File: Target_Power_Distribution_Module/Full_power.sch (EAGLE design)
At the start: 28 parts, among them IC1 MCP1702, Q1 NFET, Q2 PFET, Q3 NFET, Q4 PFET

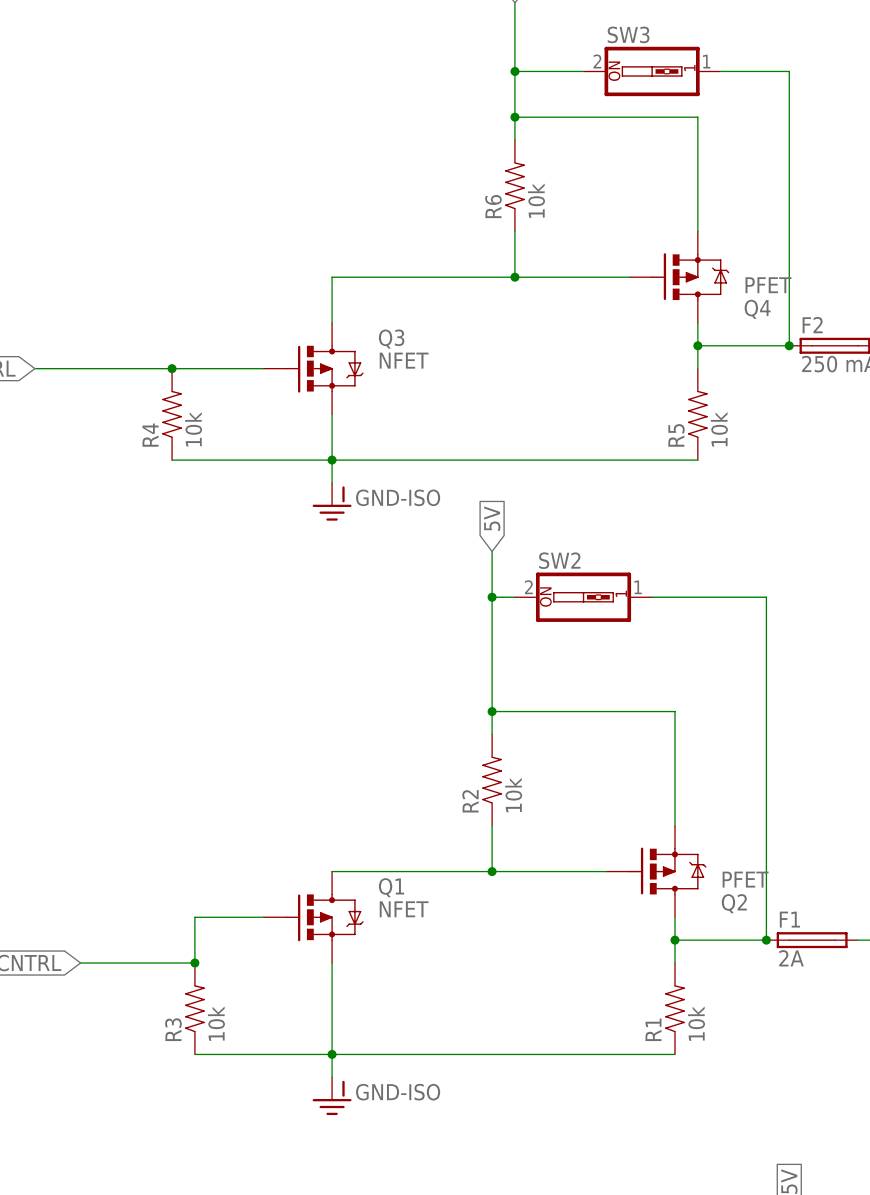
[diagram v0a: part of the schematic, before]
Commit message: Cleaned sensor on full schem
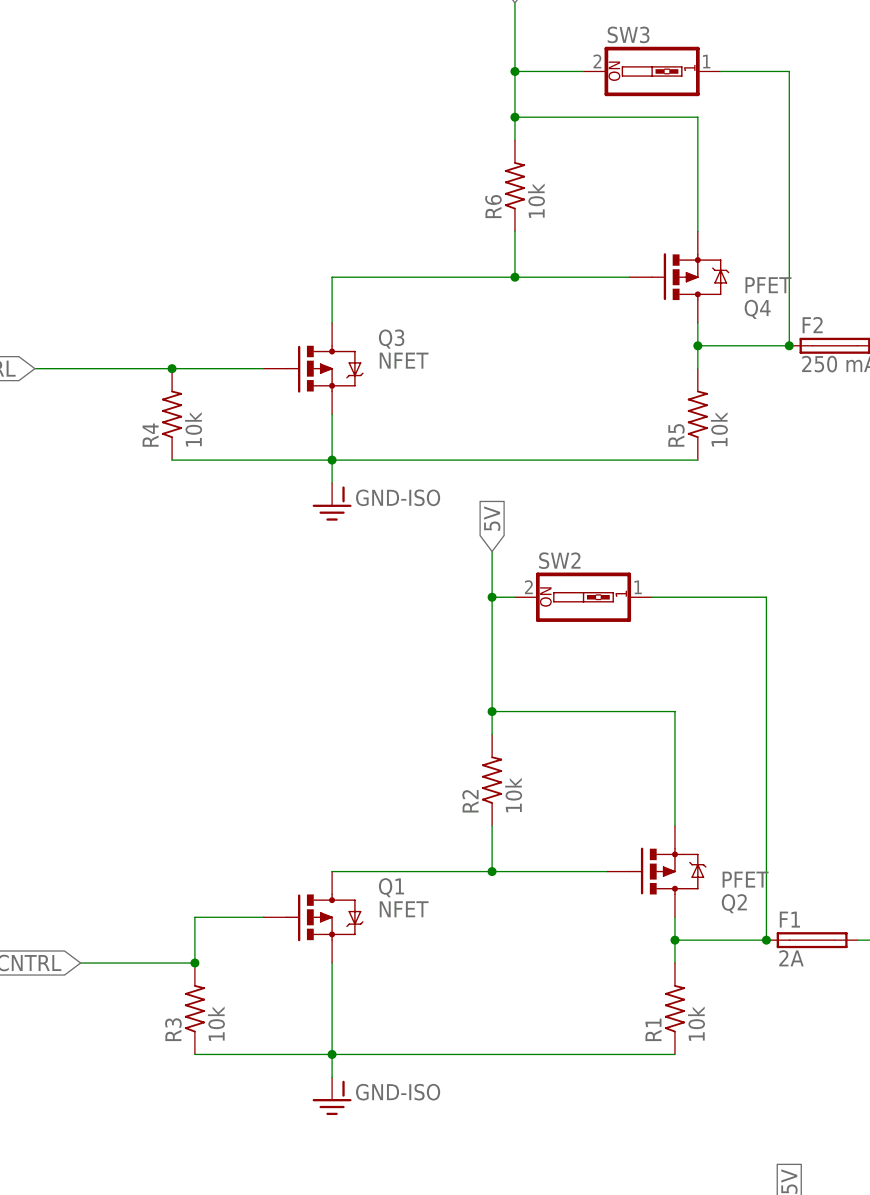
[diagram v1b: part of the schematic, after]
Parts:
- R1, R2, R3, R4, R5, R6: device SparkFun-Resistors:RESISTOR1206 -> adafruit:R-US_R1206
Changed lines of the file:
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@@
 <part name="Q2" library="User-Submitted" deviceset="MOSFET-PCHANNEL" device="FQP27P06" value="PFET"/>
 <part name="GND-ISO1" library="SparkFun-Aesthetics" deviceset="GND-ISO" device=""/>
-<part name="R1" library="SparkFun-Resistors" deviceset="RESISTOR" device="1206" value="10k"/>
-<part name="R2" library="SparkFun-Resistors" deviceset="RESISTOR" device="1206" value="10k"/>
-<part name="R3" library="SparkFun-Resistors" deviceset="RESISTOR" device="1206" value="10k"/>
+<part name="R1" library="adafruit" deviceset="R-US_" device="R1206" value="10k"/>
+<part name="R2" library="adafruit" deviceset="R-US_" device="R1206" value="10k"/>
+<part name="R3" library="adafruit" deviceset="R-US_" device="R1206" value="10k"/>
 <part name="D1" library="SparkFun-DiscreteSemi" deviceset="DIODE" device="PTH" value="1N5817"/>
 <part name="F1" library="fuse" deviceset="FUSE" device="PICOFUSE" value="2A"/>
@@
 <part name="Q4" library="User-Submitted" deviceset="MOSFET-PCHANNEL" device="FQP27P06" value="PFET"/>
 <part name="F2" library="fuse" deviceset="FUSE" device="PICOFUSE" value="250 mA"/>
-<part name="R4" library="SparkFun-Resistors" deviceset="RESISTOR" device="1206" value="10k"/>
-<part name="R5" library="SparkFun-Resistors" deviceset="RESISTOR" device="1206" value="10k"/>
-<part name="R6" library="SparkFun-Resistors" deviceset="RESISTOR" device="1206" value="10k"/>
+<part name="R4" library="adafruit" deviceset="R-US_" device="R1206" value="10k"/>
+<part name="R5" library="adafruit" deviceset="R-US_" device="R1206" value="10k"/>
+<part name="R6" library="adafruit" deviceset="R-US_" device="R1206" value="10k"/>
 <part name="GND-ISO2" library="SparkFun-Aesthetics" deviceset="GND-ISO" device=""/>
 <part name="5V_RAW1" library="SparkFun-Aesthetics" deviceset="VCC" device="" value="5V_RAW"/>
